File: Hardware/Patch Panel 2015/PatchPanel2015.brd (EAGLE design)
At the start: 209.6 x 127 mm, 55 parts

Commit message: Patch Board layout
Attempt #1 of the layout of the Patch Board
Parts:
- moved EXT_MOTOR_6 613.8 mm to (192.5, 99.3)
- moved EXT_MOTOR_5 579.2 mm to (192.3, 70.9)
- moved INT_MOTOR_6 569.9 mm to (200.2, 122.4), flipped to the bottom, turned to 180 degrees
- moved U$8 563.5 mm to (38.4, 93.2), turned to 180 degrees
- moved U$1 563.3 mm to (38.4, 82.5), turned to 180 degrees
- moved U$2 563.0 mm to (38.4, 71.9), turned to 180 degrees
- moved U$3 562.8 mm to (38.4, 61.2), turned to 180 degrees
- moved U$5 562.8 mm to (38.4, 50.8), turned to 180 degrees
- moved U$6 562.8 mm to (38.4, 40.4), turned to 180 degrees
- moved 12V_HIGH_POWER 562.5 mm to (36.6, 112.8)
- moved U$7 560.6 mm to (26.2, 99.1)
- moved EXT_MOTOR_4 545.1 mm to (192.3, 41.9)
- moved INT_MOTOR_5 536.4 mm to (199.9, 94.2), flipped to the bottom, turned to 180 degrees
- moved INT_MOTOR_4 502.5 mm to (199.9, 65.3), flipped to the bottom, turned to 180 degrees
- moved RS-485_OUT17 462.0 mm to (60.5, 115.8), turned to 180 degrees
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
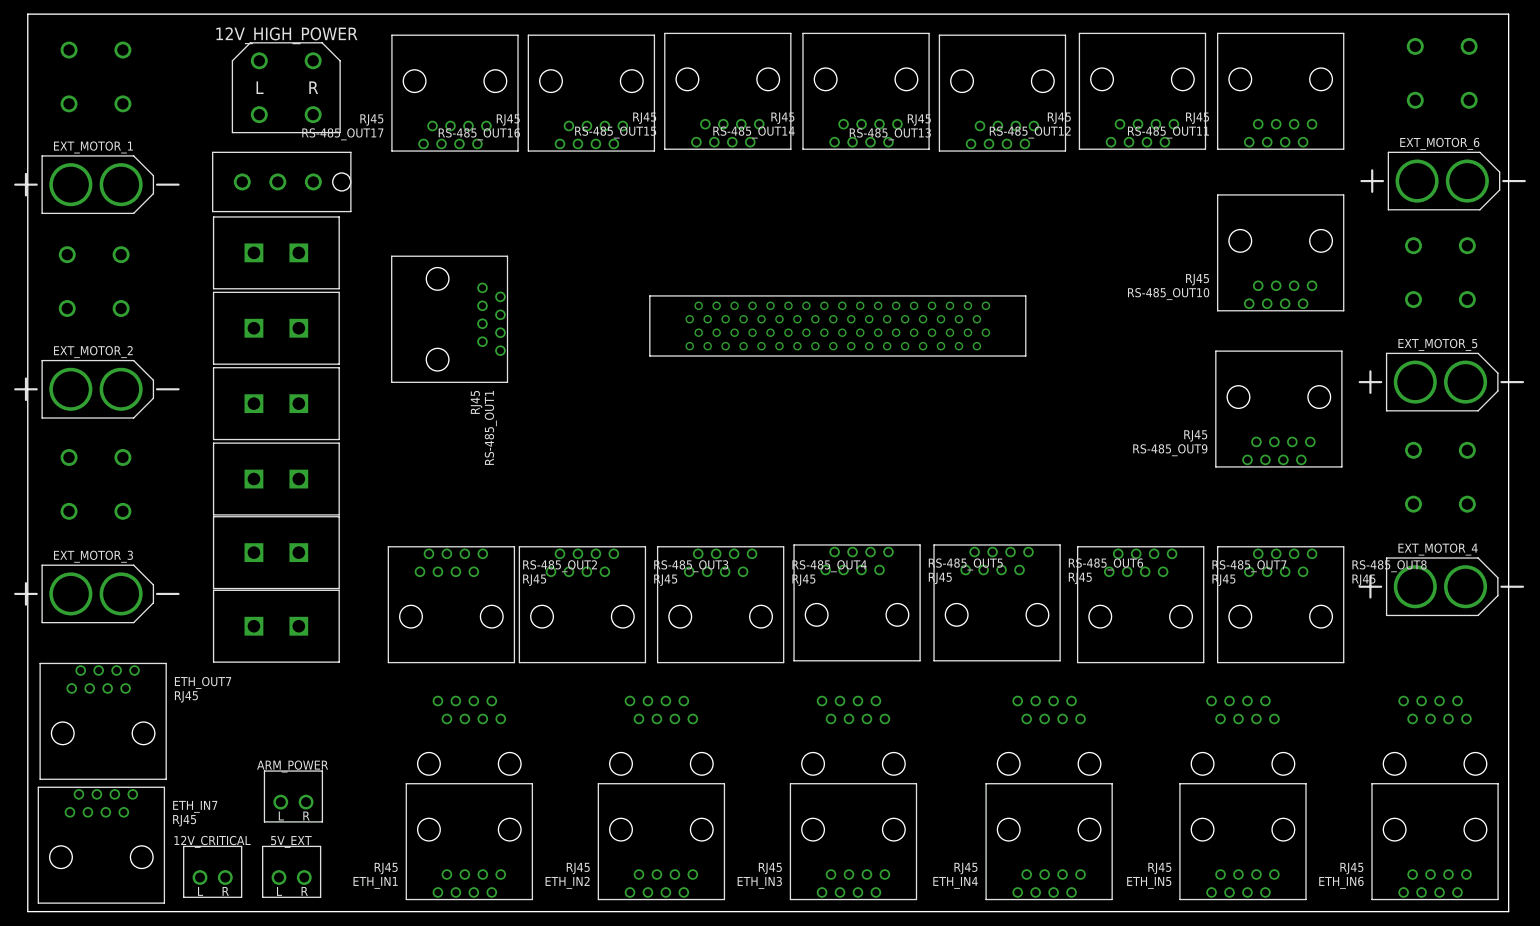
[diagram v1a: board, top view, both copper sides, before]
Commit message: Patch Board layout
layout design of the patch Board
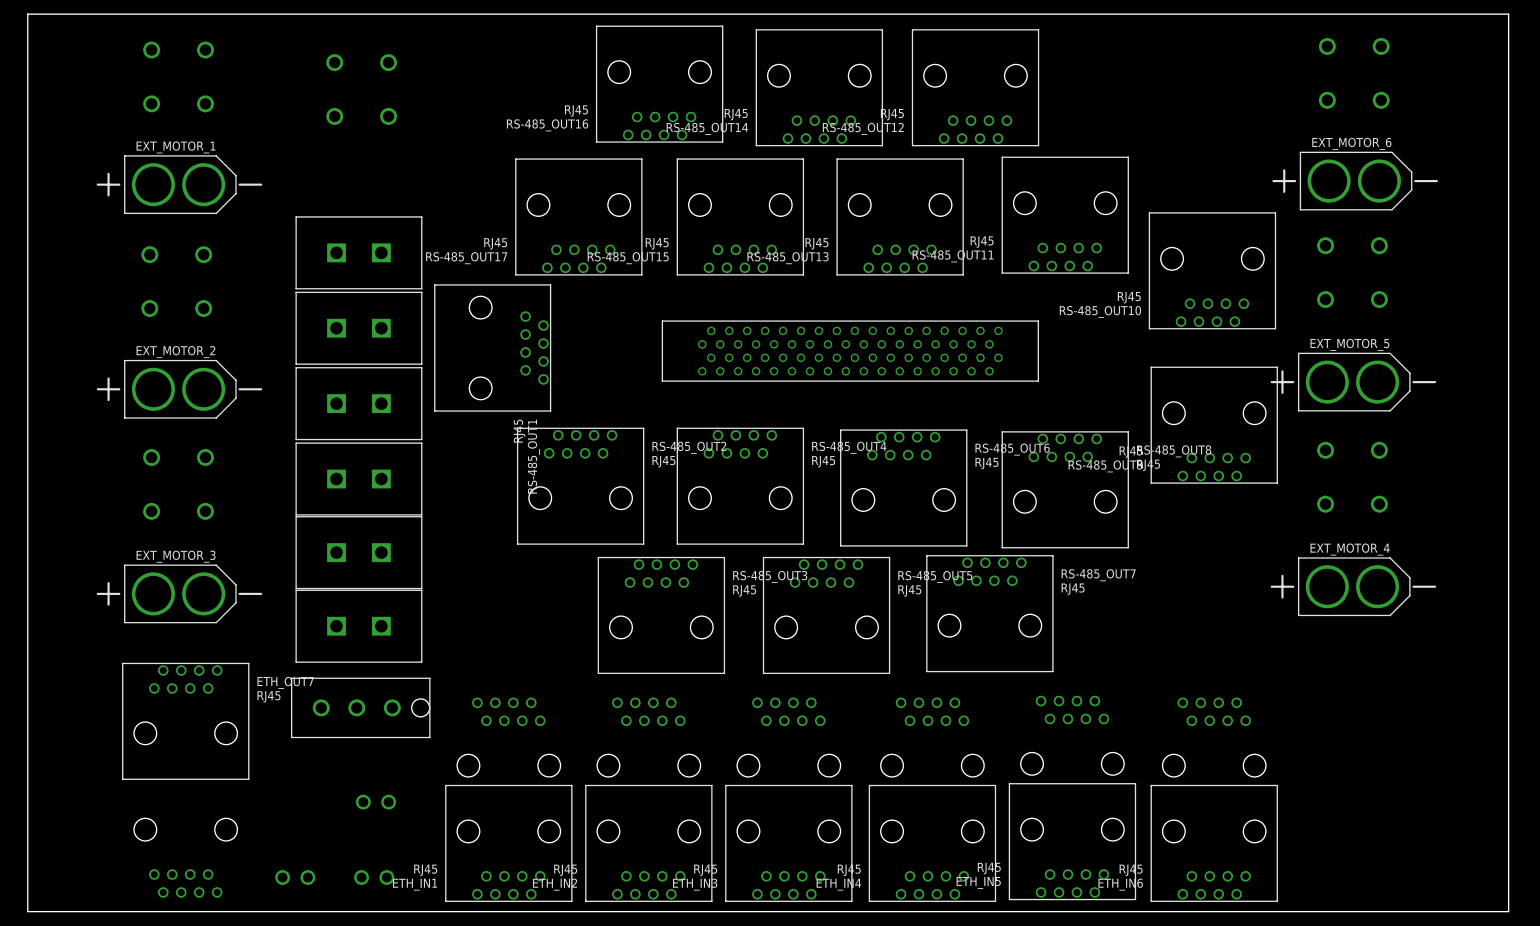
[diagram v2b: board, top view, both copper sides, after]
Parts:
- moved U$7 75.3 mm to (37.3, 24.6)
- moved RS-485_OUT11 35.2 mm to (146.8, 98.6)
- moved RS-485_OUT8 34.5 mm to (146.8, 59.7)
- moved ETH_IN6 31.2 mm to (167.9, 9.65)
- moved ETH_OUT6 31.2 mm to (167.9, 22.4)
- moved RS-485_OUT2 24.8 mm to (78.2, 60.2)
- moved RS-485_OUT17 24.8 mm to (78.0, 98.3)
- moved ETH_IN5 24.1 mm to (147.8, 9.91)
- moved ETH_OUT5 24.1 mm to (147.8, 22.6)
- moved RS-485_OUT12 23.6 mm to (134.1, 116.6)
- moved RS-485_OUT13 22.7 mm to (123.4, 98.3)
- moved RS-485_OUT7 21.4 mm to (136.1, 42.2)
- moved RS-485_OUT6 20.9 mm to (124.0, 59.9)
- moved RS-485_OUT15 17.9 mm to (100.8, 98.3)
- moved RS-485_OUT4 17.0 mm to (100.8, 60.2)
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
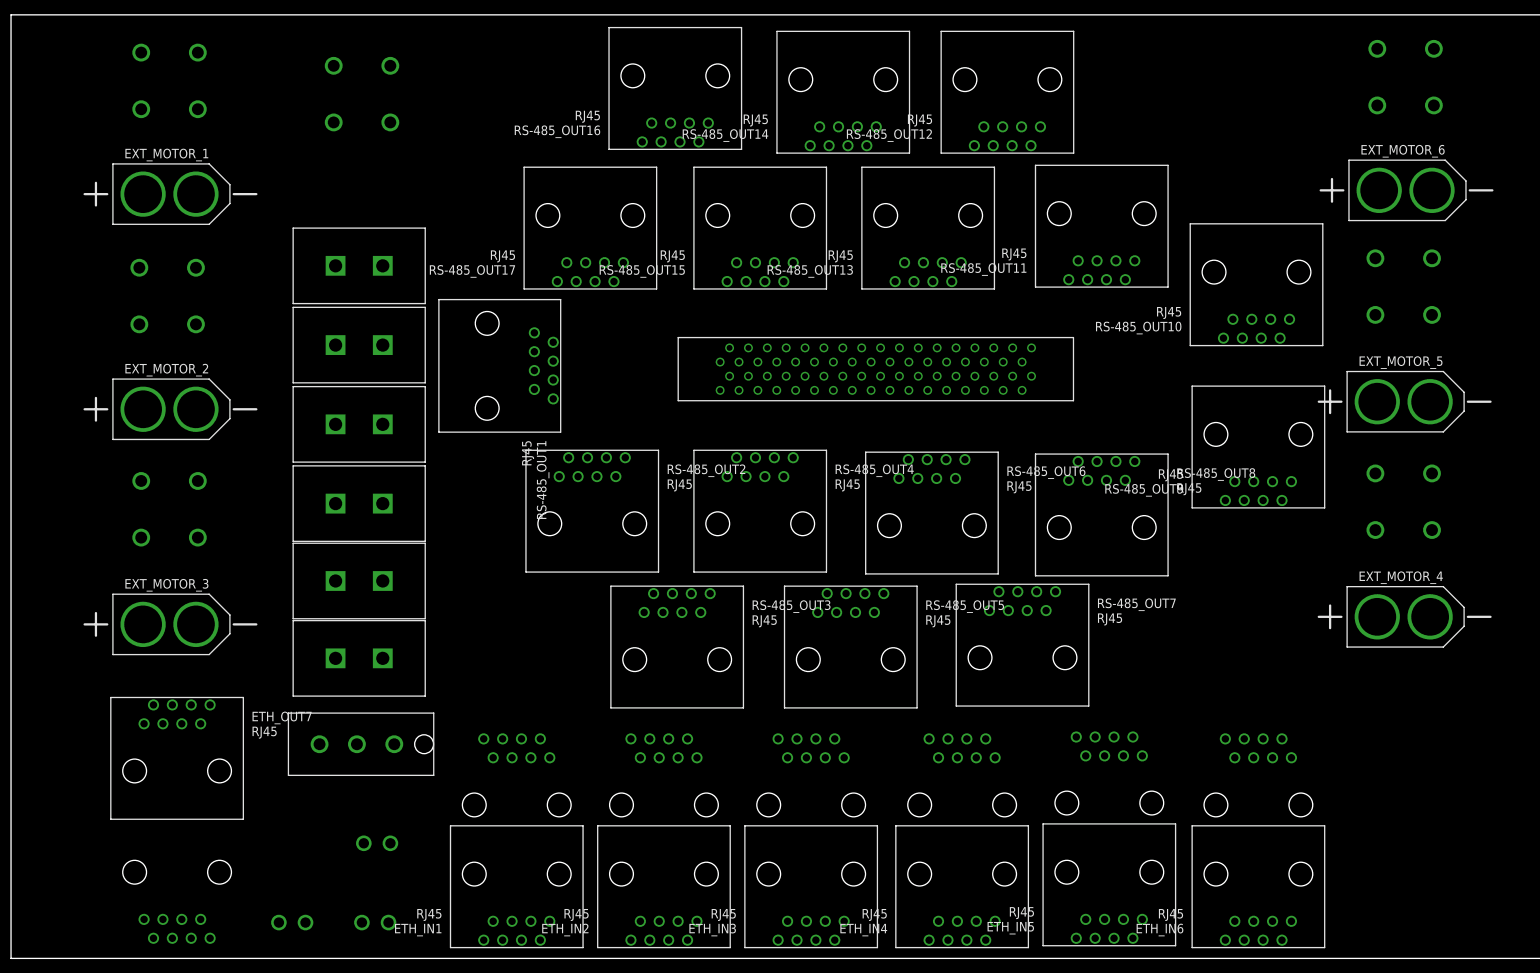
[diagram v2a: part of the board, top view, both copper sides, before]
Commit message: Patch Board Layout
Possibly final layout
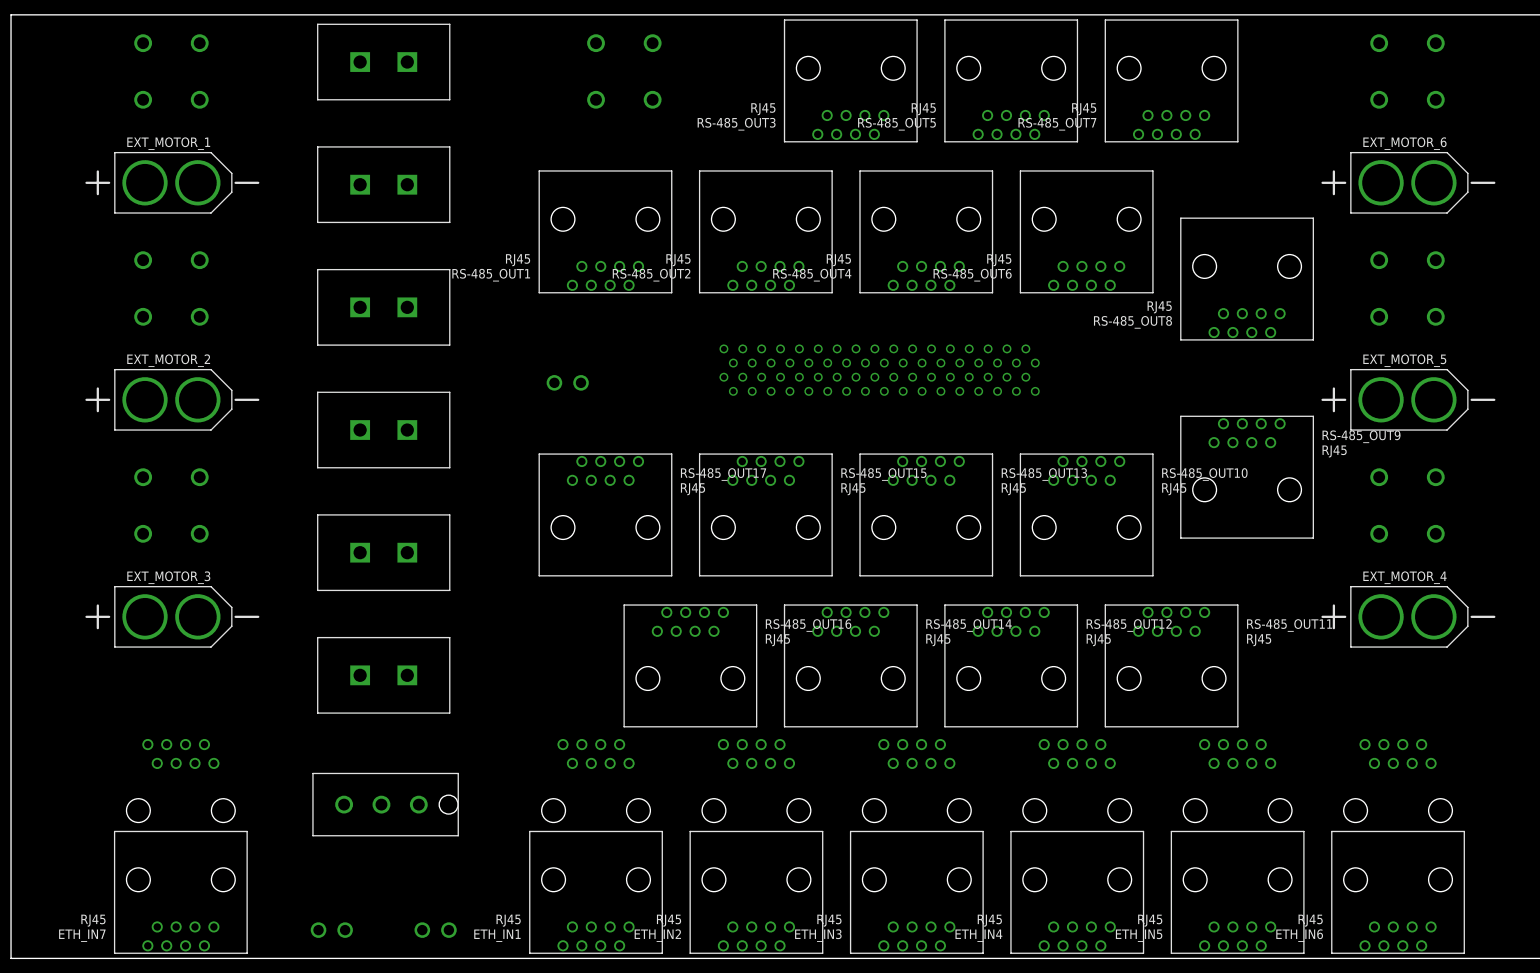
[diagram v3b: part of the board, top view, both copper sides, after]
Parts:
- moved RS-485_OUT3 79.7 mm to (113.0, 118.1), turned to 180 degrees
- moved RS-485_OUT5 79.2 mm to (134.6, 118.1), turned to 180 degrees
- moved RS-485_OUT7 78.6 mm to (156.2, 118.1), turned to 180 degrees
- moved RS-485_OUT16 77.8 mm to (91.4, 39.4), turned to 0 degrees
- moved RS-485_OUT14 77.2 mm to (113.0, 39.4), turned to 0 degrees
- moved RS-485_OUT12 77.2 mm to (134.6, 39.4), turned to 0 degrees
- moved 5V_EXT 77.1 mm to (74.9, 77.5)
- moved RS-485_OUT11 59.9 mm to (156.2, 39.4), turned to 0 degrees
- moved RS-485_OUT2 44.3 mm to (101.6, 97.8), turned to 180 degrees
- moved RS-485_OUT4 43.7 mm to (123.2, 97.8), turned to 180 degrees
- moved RS-485_OUT6 43.2 mm to (144.8, 97.8), turned to 180 degrees
- moved RS-485_OUT17 38.7 mm to (80.0, 59.7), turned to 0 degrees
- moved RS-485_OUT15 38.6 mm to (101.6, 59.7), turned to 0 degrees
- moved RS-485_OUT13 38.6 mm to (123.2, 59.7), turned to 0 degrees
- moved RS-485_OUT10 38.5 mm to (144.8, 59.7), turned to 0 degrees
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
